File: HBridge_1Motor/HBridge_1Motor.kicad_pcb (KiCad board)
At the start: 2 copper layers, 70 x 70 mm, 95 parts, among them IC1 GP1S093HCZ0F, IC2 GP1S093HCZ0F, IC3 GP1S093HCZ0F, IC4 GP1S093HCZ0F, IC5 LM393DR, IC6 MCP6002-I_SN, J1 +24V_Vin, J2 Conn_01x04_Pin, J2 MOTOR, J3 V_Motor, Q1 IRF3205SPBF, Q2 IRF3205SPBF, Q3 IRF3205SPBF, Q4 IRF3205SPBF, Q5 IRF3205SPBF, U1 AMS1117-5.0, U2 XL4015, U3 4001, U4 IR2104, U5 IR2104, U6 6N137, U7 PC817

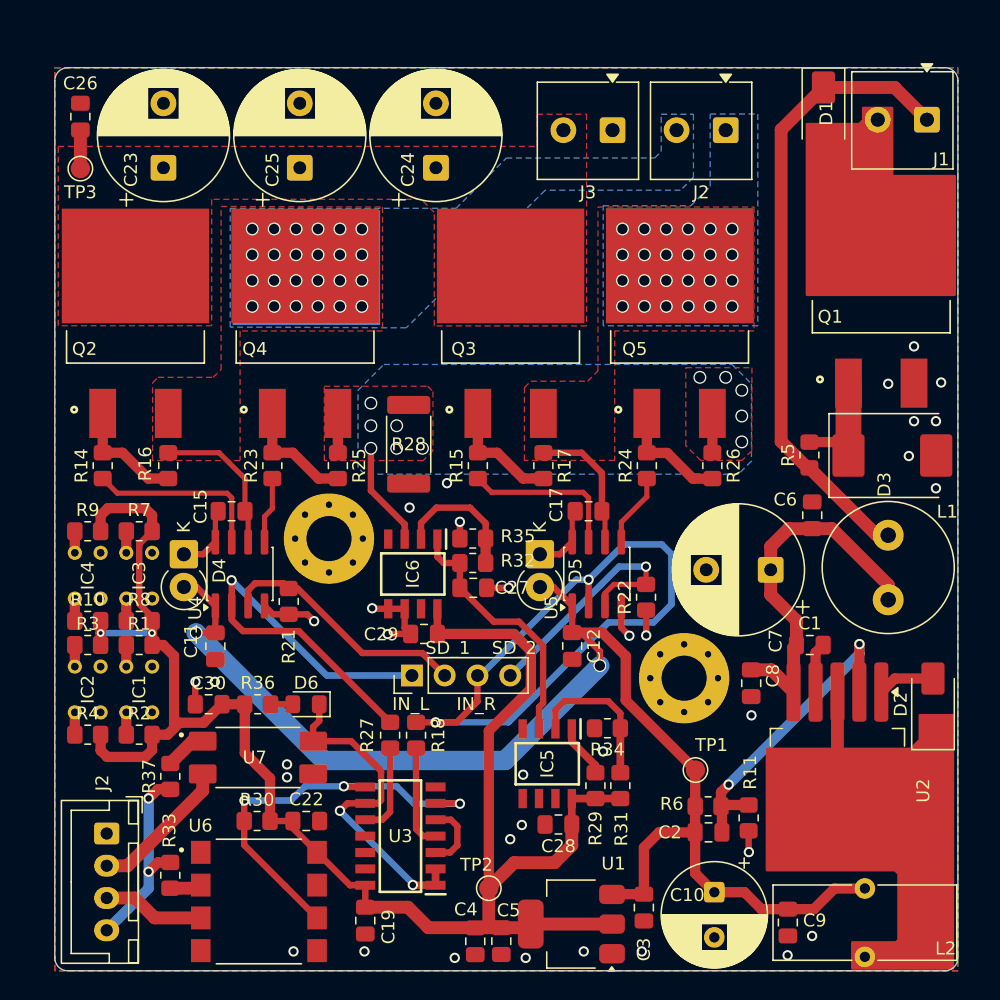
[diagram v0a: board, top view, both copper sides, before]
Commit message: edit HBridge, RTC_Pump, SmokeSensor skillscreen layers
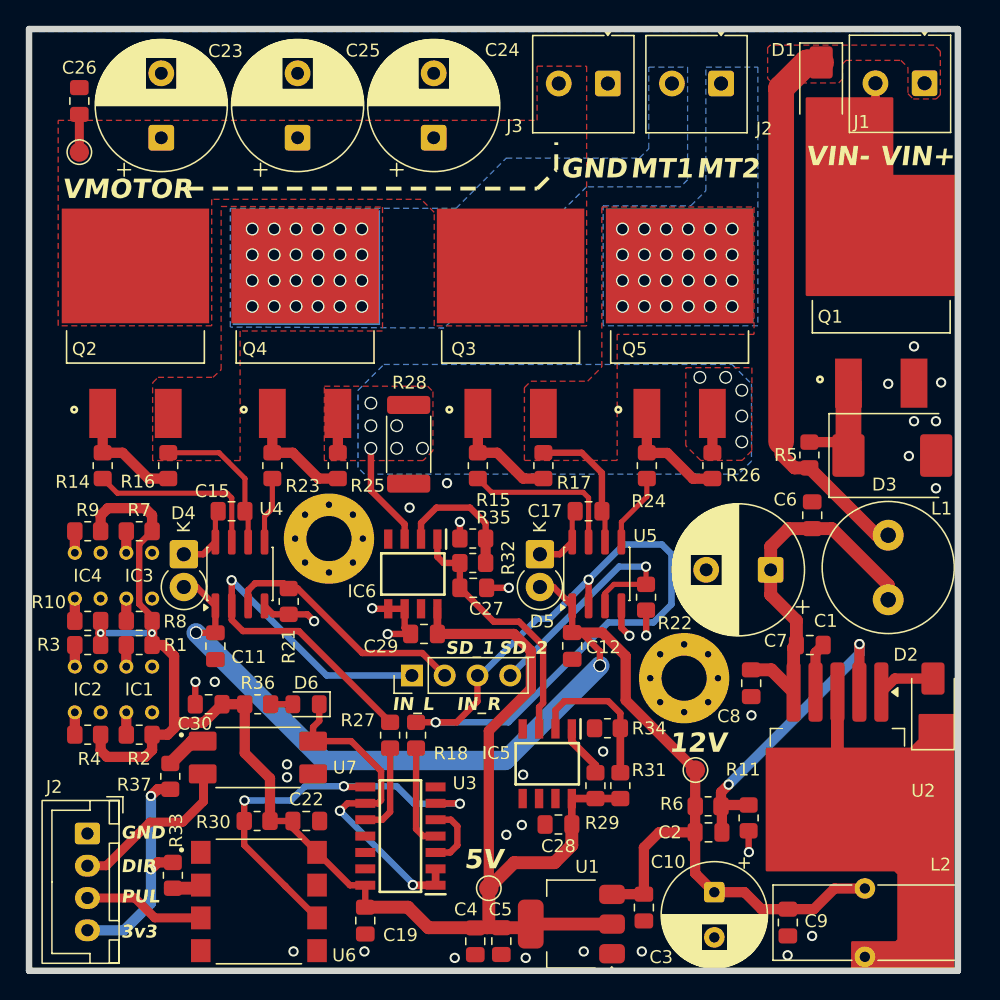
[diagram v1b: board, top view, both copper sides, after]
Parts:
- moved J2 3.64 mm to (159.8, 49.3)
- moved J3 3.64 mm to (151.0, 49.3)
- moved J1 2.84 mm to (175.5, 49.3)
- moved C24 2.33 mm to (137.5, 53.6)
- moved C23 2.33 mm to (116.4, 53.6)
- moved C25 2.33 mm to (126.9, 53.6)
- moved D1 1.95 mm to (167.5, 49.7)
- moved J2 1.49 mm to (110.6, 107.5)
- moved TP3 1.28 mm to (110.0, 54.7)
- moved C26 1.21 mm to (110.0, 50.7)
- moved R33 0.20 mm to (117.3, 110.7)
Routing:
- net Net-(D1-A1): track 49.2 -> 43.2 mm
- net DIR_MCU: track 11.2 -> 13.2 mm
- net 3v3_MCU: track 15.5 -> 17.6 mm
- net PULSE_MCU: track 7.93 -> 9.43 mm
- net Net-(D1-A2): track 4.83 -> 6.12 mm
- added copper zone on F.Cu, net Net-(D1-A1)
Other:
- board size 70 x 70 mm -> 72 x 73 mm
- board text added: "12V"
- board text added: "3v3"
- board text added: "5V"
- board text added: "DIR"
- board text added: "GND"
- board text added: "MT1"
- board text added: "MT2"
- board text added: "PUL"
- board text added: "VIN+"
- board text added: "VIN-"
- board text added: "VMOTOR"
